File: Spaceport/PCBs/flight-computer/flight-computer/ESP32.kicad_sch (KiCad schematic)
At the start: 1 part

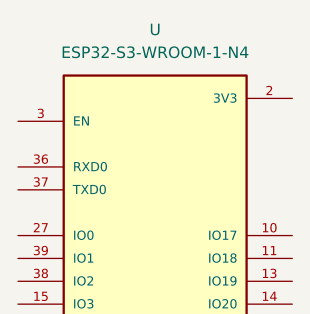
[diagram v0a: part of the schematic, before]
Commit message: Added SD Card and ESP32 UART
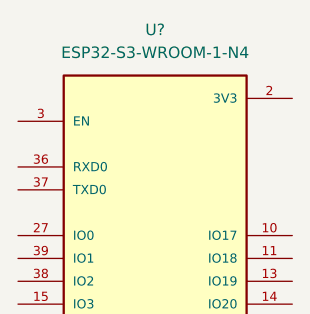
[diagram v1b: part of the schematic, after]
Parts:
- renumbered U to U?
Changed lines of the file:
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@@
 		(dnp no)
 		(fields_autoplaced yes)
-		(property "Reference" "U"
+		(property "Reference" "U?"
 			(at 147.32 49.53 0)
 			(effects
@@
 		(instances
 			(project "flight-computer"
-				(path "/b419aaf0-5349-42bc-a414-d94cafbe45e9/551958d2-abef-4077-bb30-14cb500b1ed6"
-					(reference "U8")
+				(path "/b419aaf0-5349-42bc-a414-d94cafbe45e9/cb89a847-e69c-468f-9129-87ce7a9bc840"
+					(reference "U?")
 					(unit 1)
 				)

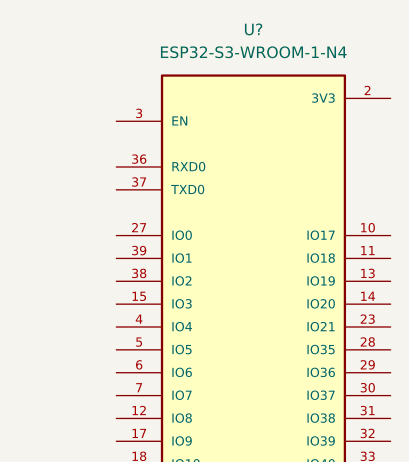
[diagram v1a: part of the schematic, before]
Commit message: added external I2C, SPI, SWD, UART connectors, cleaned up schematics, and changed STM32 schematic for one with power pins. Need to add decoupling capacitors for STM32, external clock for STM32
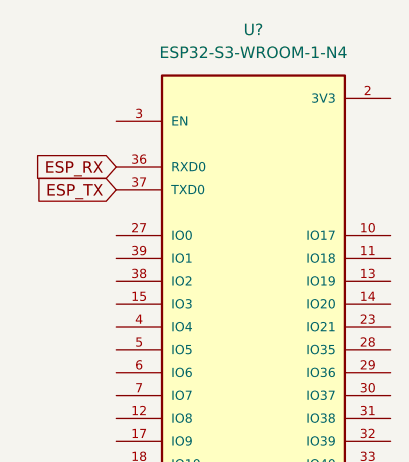
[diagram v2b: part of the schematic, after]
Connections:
- net ESP_RX: now reaches U?.36 (RXD0)
- net ESP_TX: now reaches U?.37 (TXD0)
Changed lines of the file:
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@@
 	(generator_version "9.0")
 	(paper "A4")
+	(global_label "ESP_RX"
+		(shape input)
+		(at 132.08 64.77 180)
+		(fields_autoplaced yes)
+		(effects
+			(font
+				(size 1.27 1.27)
+			)
+			(justify right)
+		)
+		(property "Intersheetrefs" "${INTERSHEET_REFS}"
+			(at 122.0192 64.77 0)
+			(effects
+				(font
+					(size 1.27 1.27)
+				)
+				(justify right)
+				(hide yes)
+			)
+		)
+	)
+	(global_label "ESP_TX"
+		(shape input)
+		(at 132.08 67.31 180)
+		(fields_autoplaced yes)
+		(effects
+			(font
+				(size 1.27 1.27)
+			)
+			(justify right)
+		)
+		(property "Intersheetrefs" "${INTERSHEET_REFS}"
+			(at 122.3216 67.31 0)
+			(effects
+				(font
+					(size 1.27 1.27)
+				)
+				(justify right)
+				(hide yes)
+			)
+		)
+	)
 	(symbol
 		(lib_id "SRAD-Avionics:ESP32-S3-WROOM-1-N4")

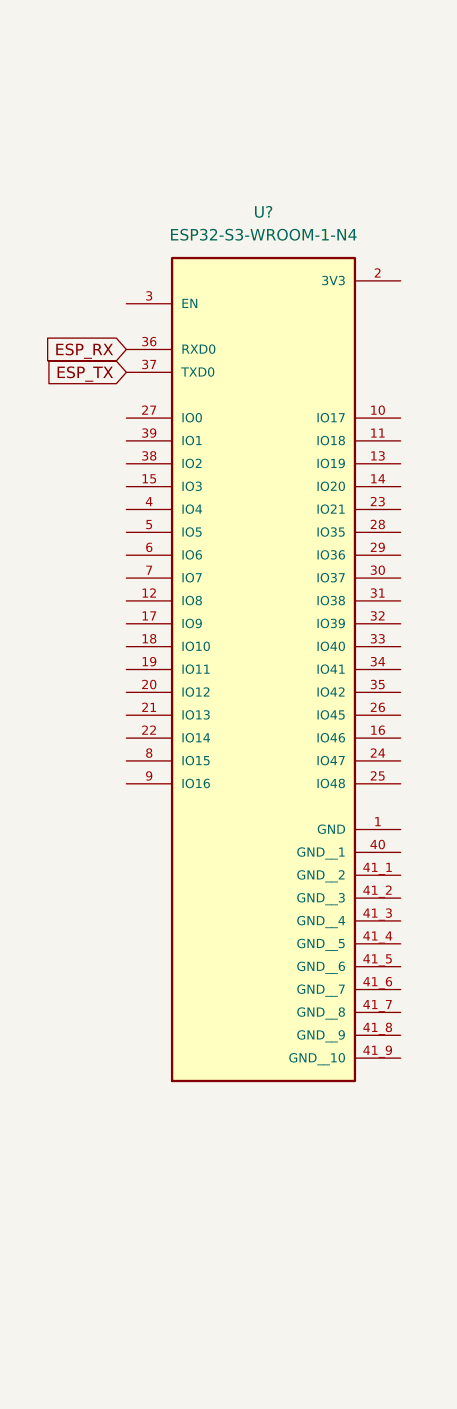
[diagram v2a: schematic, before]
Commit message: Added LEDS, Buzzer, Oscillator, decoupling capacitors, fixed 3.3 volt netclasses, reorganized main schematic page, added some annotations
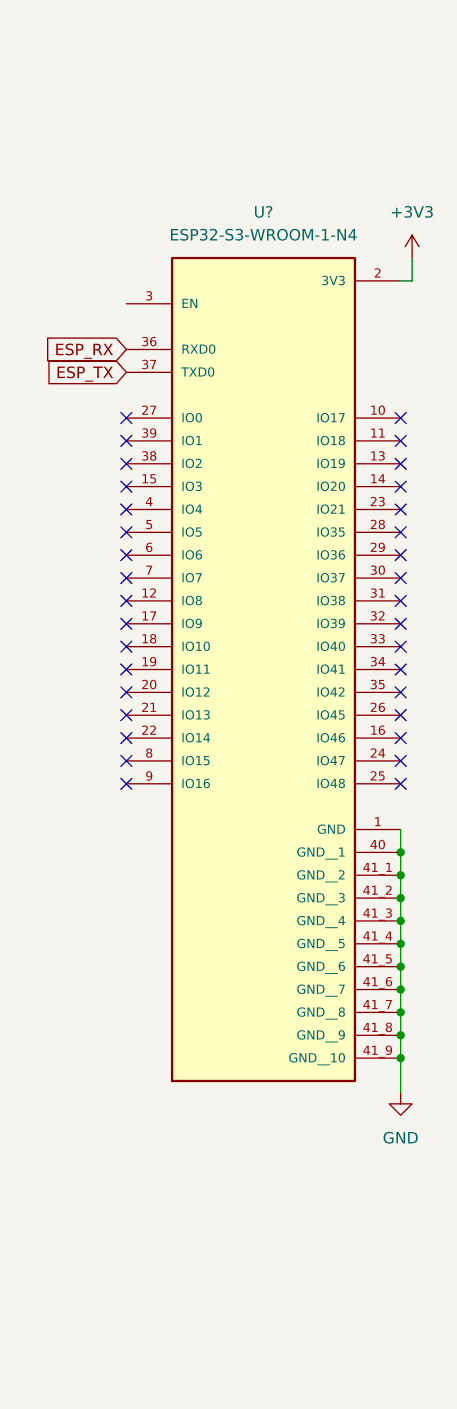
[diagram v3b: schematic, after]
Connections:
- net GND: now reaches U?.1 (GND)
- net GND: now also U?.40 (GND__1), U?.41_1 (GND__2), U?.41_2 (GND__3), U?.41_3 (GND__4), U?.41_4 (GND__5), U?.41_5 (GND__6), U?.41_6 (GND__7), U?.41_7 (GND__8), U?.41_8 (GND__9), U?.41_9 (GND__10)
- net +3V3: now reaches U?.2 (3V3)
- no-connect marks 0 -> 34

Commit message: swich ESP32 to for ESP32-S3-MINI because that is the on we are ordeirng
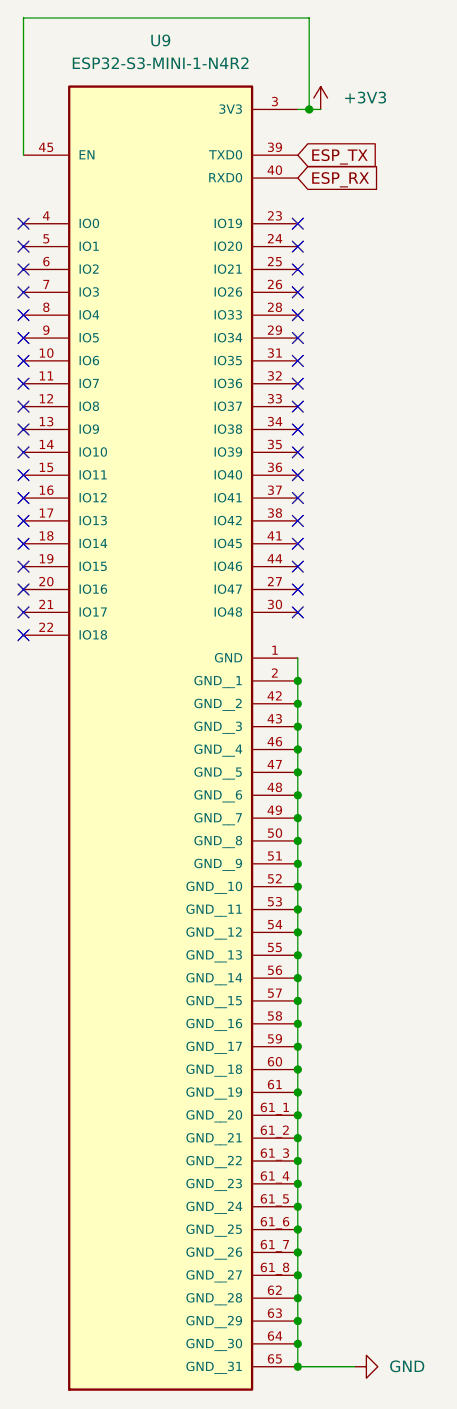
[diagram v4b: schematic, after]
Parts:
- removed U?: ESP32-S3-WROOM-1-N4, ESP32-S3-WROOM-1-N4:XCVR_ESP32-S3-WROOM-1-N4, symbol SRAD-Avionics:ESP32-S3-WROOM-1-N4
- added U9: ESP32-S3-MINI-1-N4R2, ESP32-S3-MINI-1-N4R2:XCVR_ESP32-S3-MINI-1-N4R2, symbol SRAD-Avionics:ESP32-S3-MINI-1-N4R2
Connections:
- net +3V3: now also U9.3 (3V3), U9.45 (EN)
- net ESP_RX: now also U9.40 (RXD0)
- net ESP_TX: now also U9.39 (TXD0)
- net GND: now also U9.1 (GND), U9.2 (GND__1), U9.42 (GND__2), U9.43 (GND__3), U9.46 (GND__4), U9.47 (GND__5), U9.48 (GND__6), U9.49 (GND__7), U9.50 (GND__8), U9.51 (GND__9), U9.52 (GND__10), U9.53 (GND__11), U9.54 (GND__12), U9.55 (GND__13), U9.56 (GND__14), U9.57 (GND__15), U9.58 (GND__16), U9.59 (GND__17), U9.60 (GND__18), U9.61 (GND__19), U9.61_1 (GND__20), U9.61_2 (GND__21), U9.61_3 (GND__22), U9.61_4 (GND__23), U9.61_5 (GND__24), U9.61_6 (GND__25), U9.61_7 (GND__26), U9.61_8 (GND__27), U9.62 (GND__28), U9.63 (GND__29), U9.64 (GND__30), U9.65 (GND__31)
- no-connect marks 34 -> 37
